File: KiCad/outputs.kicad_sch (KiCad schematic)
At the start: 32 parts, among them J1 UART, J10 LED2, J13 LED3, J14 LED4, J15 LED8, J16 LED7, J17 LED6, J18 LED5, J19 LED9, J2 VDD, J20 LED10, J21 LED11, J22 LED12, J3 GND, J6 USB_C_Receptacle_USB2.0_16P, J7 Conn_01x14, J8 JTAG, J9 LED1, U7 SN74LVC8T245, U8 SN74LVC8T245

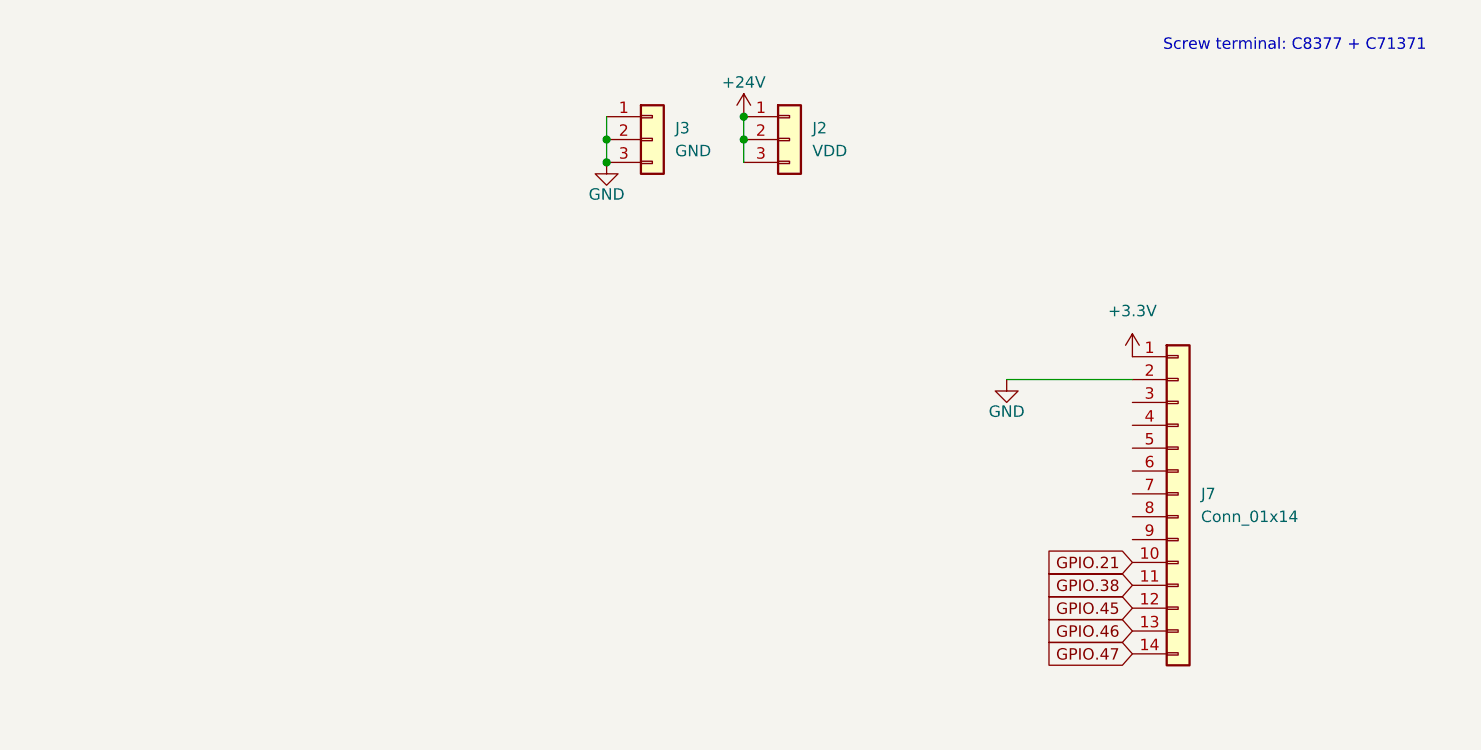
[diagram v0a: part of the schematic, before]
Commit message: work
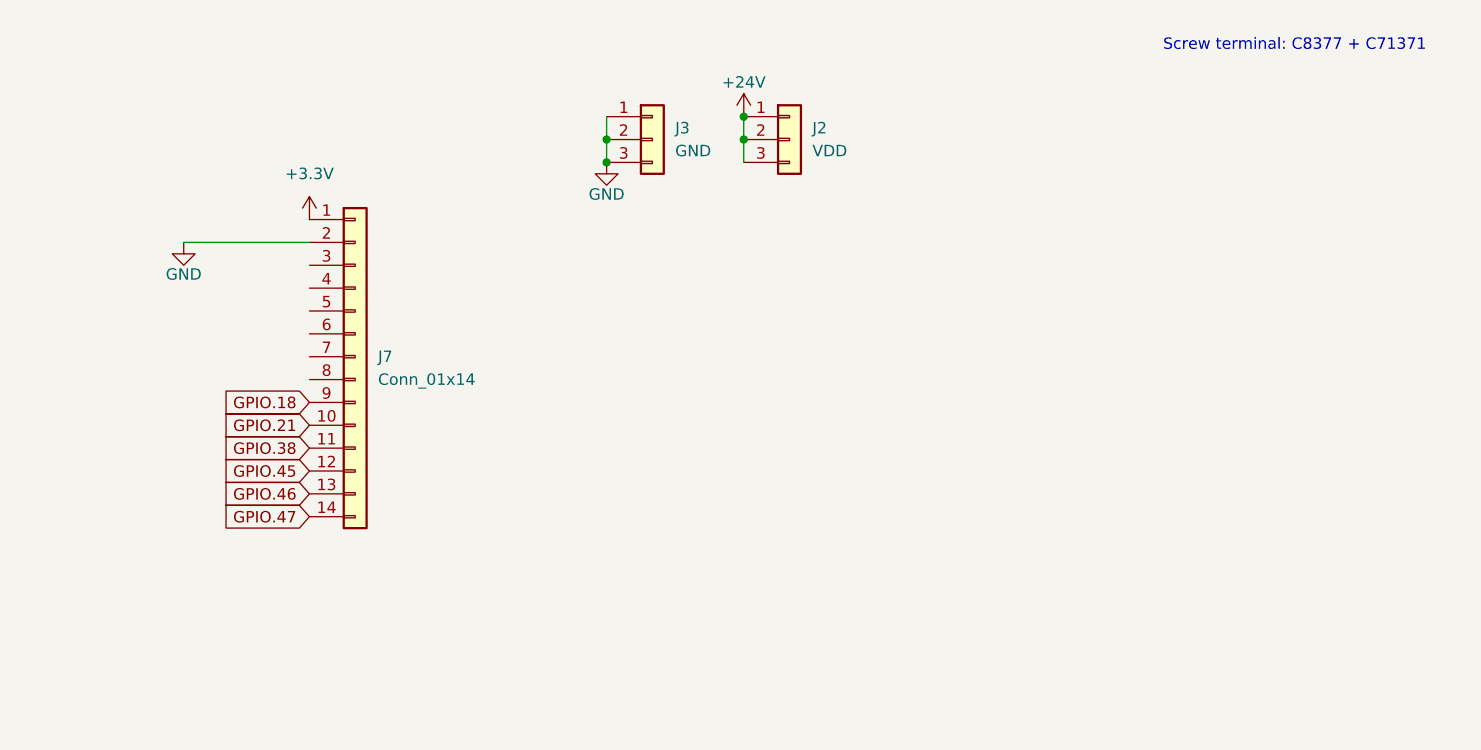
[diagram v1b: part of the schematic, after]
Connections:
- net GPIO.18: now reaches J7.9 (Pin_9)
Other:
- moved on the sheet: J7
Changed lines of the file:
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@@
 	(wire
 		(pts
-			(xy 189.23 127) (xy 203.2 127)
+			(xy 97.79 111.76) (xy 111.76 111.76)
 		)
 		(stroke
@@
 	(global_label "GPIO.45"
 		(shape input)
-		(at 203.2 152.4 180)
+		(at 111.76 137.16 180)
 		(fields_autoplaced yes)
 		(effects
@@
 		)
 		(property "Intersheetrefs" "${INTERSHEET_REFS}"
-			(at 192.7157 152.4 0)
+			(at 101.2757 137.16 0)
 			(hide yes)
 			(show_name no)
@@
 	(global_label "GPIO.21"
 		(shape input)
-		(at 203.2 147.32 180)
+		(at 111.76 132.08 180)
 		(fields_autoplaced yes)
 		(effects
@@
 		)
 		(property "Intersheetrefs" "${INTERSHEET_REFS}"
-			(at 192.7157 147.32 0)
+			(at 101.2757 132.08 0)
 			(hide yes)
 			(show_name no)
@@
 	(global_label "GPIO.47"
 		(shape input)
-		(at 203.2 157.48 180)
+		(at 111.76 142.24 180)
 		(fields_autoplaced yes)
 		(effects
@@
 		)
 		(property "Intersheetrefs" "${INTERSHEET_REFS}"
-			(at 192.7157 157.48 0)
+			(at 101.2757 142.24 0)
 			(hide yes)
 			(show_name no)
@@
 	(global_label "GPIO.46"
 		(shape input)
-		(at 203.2 154.94 180)
+		(at 111.76 139.7 180)
 		(fields_autoplaced yes)
 		(effects
@@
 		)
 		(property "Intersheetrefs" "${INTERSHEET_REFS}"
-			(at 192.7157 154.94 0)
+			(at 101.2757 139.7 0)
 			(hide yes)
 			(show_name no)
@@
 		)
 	)
+	(global_label "GPIO.18"
+		(shape input)
+		(at 111.76 129.54 180)
+		(fields_autoplaced yes)
+		(effects
+			(font
+				(size 1.27 1.27)
+			)
+			(justify right)
+		)
+		(property "Intersheetrefs" "${INTERSHEET_REFS}"
+			(at 101.2757 129.54 0)
+			(hide yes)
+			(show_name no)
+			(do_not_autoplace no)
+			(effects
+				(font
+					(size 1.27 1.27)
+				)
+				(justify right)
+			)
+		)
+	)
 	(global_label "DataOut2"
 		(shape input)
@@
 	(global_label "GPIO.38"
 		(shape input)
-		(at 203.2 149.86 180)
+		(at 111.76 134.62 180)
 		(fields_autoplaced yes)
 		(effects
@@
 		)
 		(property "Intersheetrefs" "${INTERSHEET_REFS}"
-			(at 192.7157 149.86 0)
+			(at 101.2757 134.62 0)
 			(hide yes)
 			(show_name no)
@@
 	(symbol
 		(lib_id "Connector_Generic:Conn_01x14")
-		(at 208.28 139.7 0)
+		(at 116.84 124.46 0)
 		(unit 1)
 		(body_style 1)
@@
 		(fields_autoplaced yes)
 		(property "Reference" "J7"
-			(at 210.82 139.6999 0)
+			(at 119.38 124.4599 0)
 			(show_name no)
 			(do_not_autoplace no)
@@
 		)
 		(property "Value" "Conn_01x14"
-			(at 210.82 142.2399 0)
+			(at 119.38 126.9999 0)
 			(show_name no)
 			(do_not_autoplace no)
@@
 		)
 		(property "Footprint" "Connector_PinHeader_2.54mm:PinHeader_1x14_P2.54mm_Vertical"
-			(at 208.28 139.7 0)
+			(at 116.84 124.46 0)
 			(hide yes)
 			(show_name no)
@@
 		)
 		(property "Datasheet" ""
-			(at 208.28 139.7 0)
+			(at 116.84 124.46 0)
 			(hide yes)
 			(show_name no)
@@
 		)
 		(property "Description" "Generic connector, single row, 01x14, script generated (kicad-library-utils/schlib/autogen/connector/)"
-			(at 208.28 139.7 0)
+			(at 116.84 124.46 0)
 			(hide yes)
 			(show_name no)
@@
 		)
 		(property "LCSC" ""
-			(at 208.28 139.7 0)
+			(at 116.84 124.46 0)
 			(hide yes)
 			(show_name no)
@@
 	(symbol
 		(lib_id "power:GND")
-		(at 189.23 127 0)
+		(at 97.79 111.76 0)
 		(unit 1)
 		(body_style 1)
@@
 		(dnp no)
 		(property "Reference" "#PWR012"
-			(at 189.23 133.35 0)
+			(at 97.79 118.11 0)
 			(hide yes)
 			(show_name no)
@@
 		)
 		(property "Value" "GND"
-			(at 189.23 130.556 0)
+			(at 97.79 115.316 0)
 			(show_name no)
 			(do_not_autoplace no)
@@
 		)
 		(property "Footprint" ""
-			(at 189.23 127 0)
+			(at 97.79 111.76 0)
 			(hide yes)
 			(show_name no)
@@
 		)
 		(property "Datasheet" ""
-			(at 189.23 127 0)
+			(at 97.79 111.76 0)
 			(hide yes)
 			(show_name no)
@@
 		)
 		(property "Description" "Power symbol creates a global label with name \"GND\" , ground"
-			(at 189.23 127 0)
+			(at 97.79 111.76 0)
 			(hide yes)
 			(show_name no)
@@
 	(symbol
 		(lib_id "power:+3.3V")
-		(at 203.2 124.46 0)
+		(at 111.76 109.22 0)
 		(unit 1)
 		(body_style 1)
@@
 		(dnp no)
 		(property "Reference" "#PWR011"
-			(at 203.2 128.27 0)
+			(at 111.76 113.03 0)
 			(hide yes)
 			(show_name no)
@@
 		)
 		(property "Value" "+3.3V"
-			(at 203.2 119.38 0)
+			(at 111.76 104.14 0)
 			(show_name no)
 			(do_not_autoplace no)
@@
 		)
 		(property "Footprint" ""
-			(at 203.2 124.46 0)
+			(at 111.76 109.22 0)
 			(hide yes)
 			(show_name no)
@@
 		)
 		(property "Datasheet" ""
-			(at 203.2 124.46 0)
+			(at 111.76 109.22 0)
 			(hide yes)
 			(show_name no)
@@
 		)
 		(property "Description" "Power symbol creates a global label with name \"+3.3V\""
-			(at 203.2 124.46 0)
+			(at 111.76 109.22 0)
 			(hide yes)
 			(show_name no)
